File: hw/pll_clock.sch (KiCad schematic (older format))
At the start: 21 parts, among them J7 BNC, U7 5P49V5925, Y1 25MHz

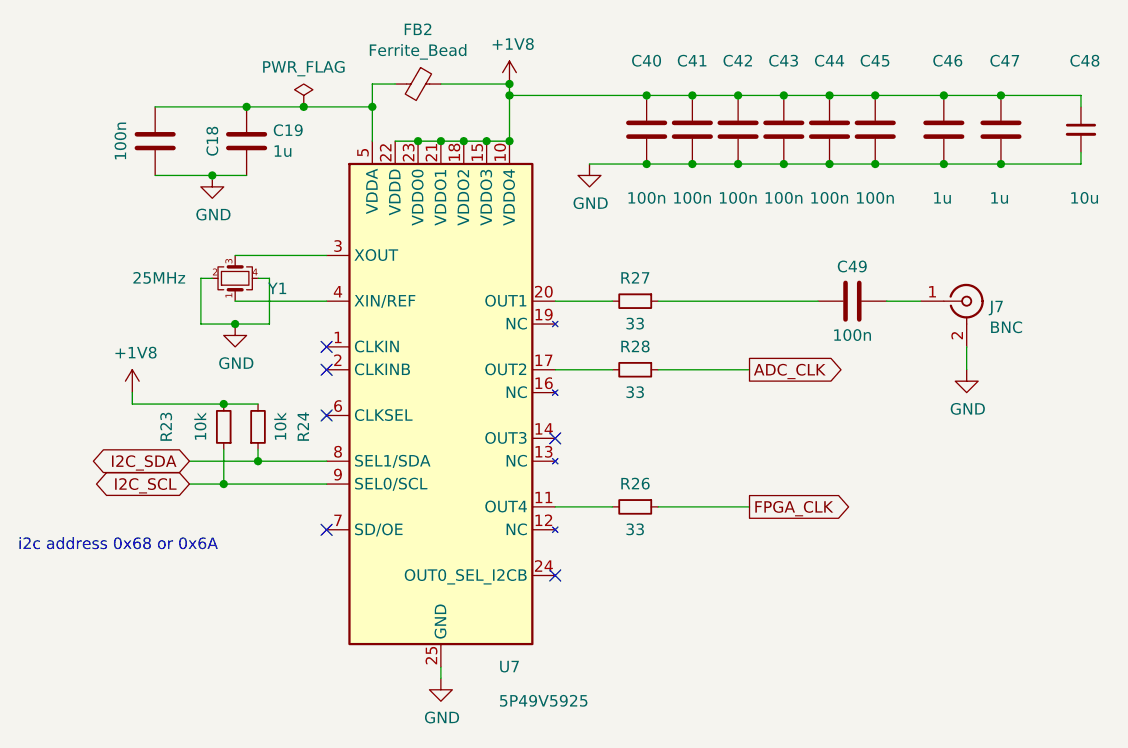
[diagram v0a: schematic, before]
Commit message: more work (don't recall details :-()
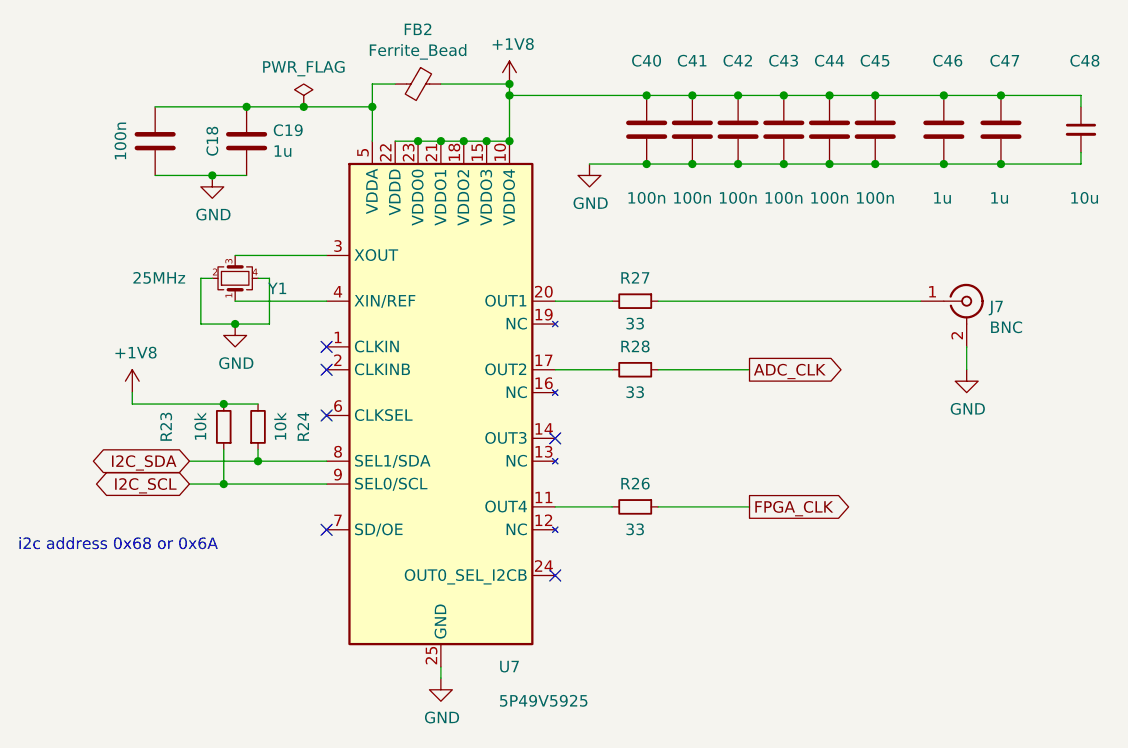
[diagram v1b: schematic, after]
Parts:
- removed C49: 100n, Capacitor_SMD:C_0603_1608Metric, symbol fmc:100nF_603
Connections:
- net at R27.1: now also J7.1 (In)
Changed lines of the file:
@@
 	1    0    0    -1
 $EndComp
-$Comp
-L fmc:100nF_603 C?
-U 1 1 60B85B4A
-P 7400 2900
-AR Path="/6086F2E3/60B85B4A" Ref="C?"  Part="1"
-AR Path="/60B16D71/60B85B4A" Ref="C49"  Part="1"
-F 0 "C49" V 7550 2900 50  0000 C CNN
-F 1 "100n" V 7250 2900 50  0000 C CNN
-F 2 "Capacitor_SMD:C_0603_1608Metric" H 7438 2750 50  0001 C CNN
-F 3 "~" H 7400 2900 50  0001 C CNN
-F 4 "GCJ188R71E104KA12D" H 7525 3100 50  0001 C CNN "Part"
-F 5 "Murata" H 7625 3200 50  0001 C CNN "Manufacturer"
-	1    7400 2900
-	0    -1   -1   0
-$EndComp
-Wire Wire Line
-	7550 2900 7700 2900
 Wire Wire Line
 	5500 2200 5600 2200
@@
 	6550 3200 6950 3200
 Wire Wire Line
-	6550 2900 7250 2900
-Wire Wire Line
 	7900 3100 7900 3200
 Text Notes 3750 4000 0    50   ~ 0
 i2c address 0x68 or 0x6A
+Wire Wire Line
+	6550 2900 7700 2900
 $EndSCHEMATC
